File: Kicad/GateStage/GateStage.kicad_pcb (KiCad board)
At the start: 2 copper layers, 66.7 x 41.9 mm, 28 parts, among them J1 Conn_01x04, J2 Conn_01x02, J3 Conn_01x03, Q1 PHP23NQ11T,127, Q2 PHP23NQ11T,127, Q3 PHP23NQ11T,127, Q4 PHP23NQ11T,127, U1 DGD05463FN-7, U2 DGD05463FN-7

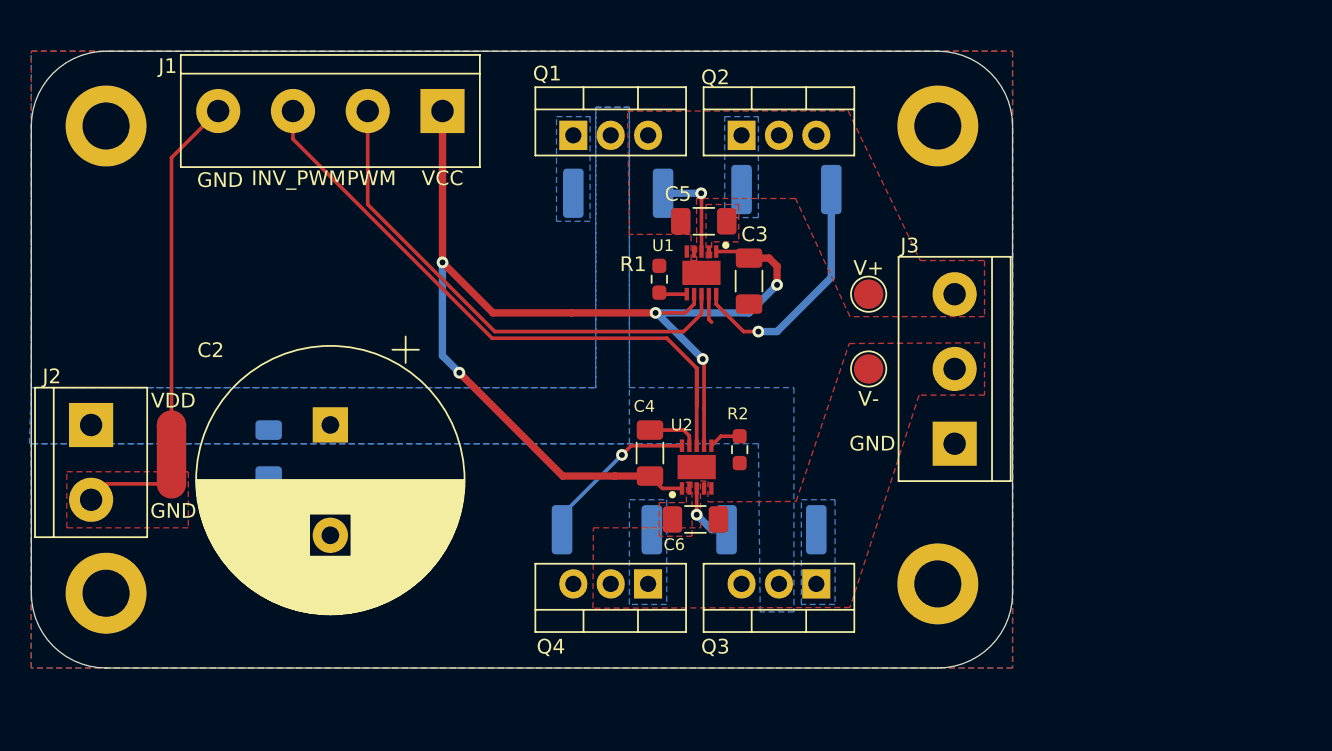
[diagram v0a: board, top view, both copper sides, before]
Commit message: Redo GateStage Board
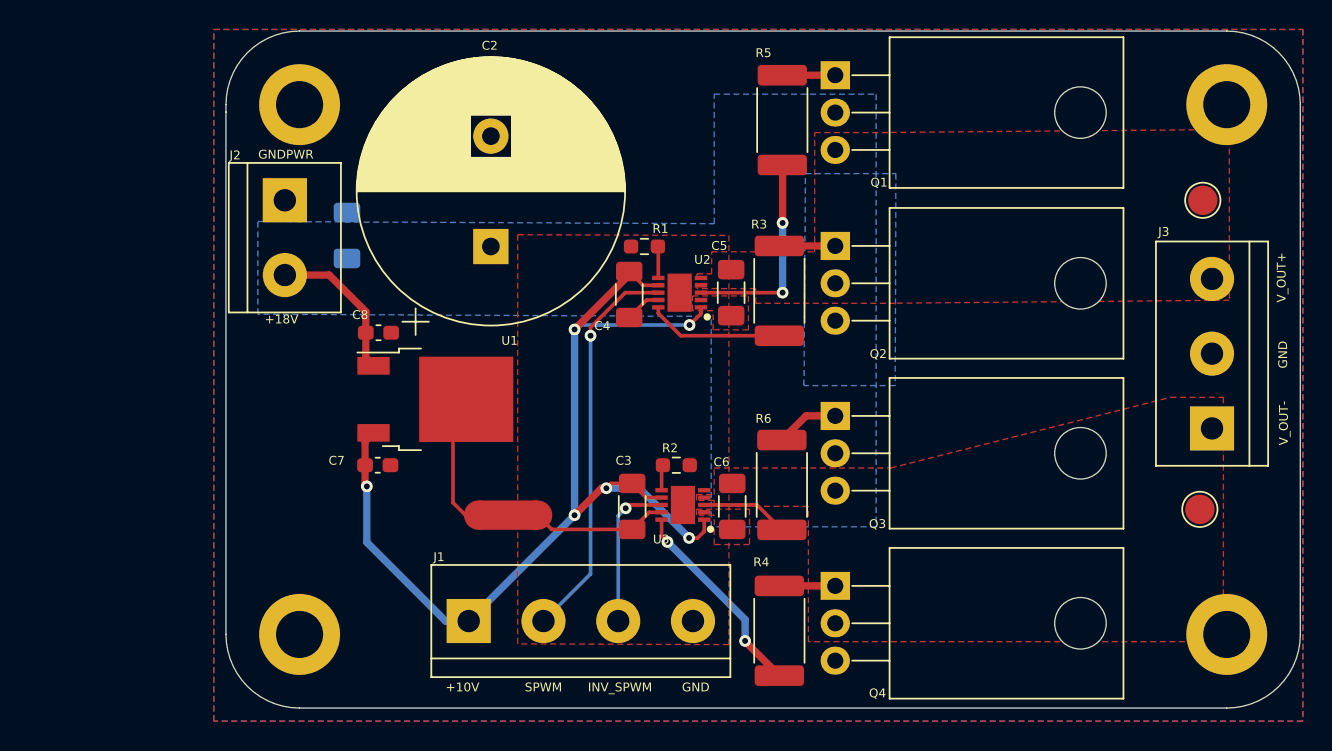
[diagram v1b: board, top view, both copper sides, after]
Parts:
- removed TPe: TestPoint, TestPoint:TestPoint_Pad_D2.0mm
- added C7: 100n, Capacitor_SMD:C_0603_1608Metric_Pad1.08x0.95mm_HandSolder, F.Cu at (125.1, 58.6)
- added C8: 330n, Capacitor_SMD:C_0603_1608Metric_Pad1.08x0.95mm_HandSolder, F.Cu at (125.2, 49.6)
- added TP2: TestPoint, TestPoint:TestPoint_Pad_D2.0mm, F.Cu at (181.0, 61.6)
- added U3: DGD05463FN-7, DGD05463:SON50P300X300X80-11N-D, F.Cu at (145.9, 61.3)
- Q1, Q2, Q3, Q4: footprint Package_TO_SOT_THT:TO-220-3_Vertical -> Package_TO_SOT_THT:TO-220-3_Horizontal_TabDown
- R3, R4, R5, R6: moved to F.Cu
- U1: value DGD05463FN-7 -> L78M10ABDT; footprint DGD05463:SON50P300X300X80-11N-D -> Package_TO_SOT_SMD:TO-252-2
- moved H2 76.2 mm to (182.8, 34.1)
- moved H1 43.4 mm to (119.8, 34.1)
- moved J1 34.7 mm to (131.3, 69.2), turned to 0 degrees
- moved TP1 23.6 mm to (181.2, 40.6)
- moved NT1 23.2 mm to (134.0, 62.0), turned to 180 degrees
- moved J2 20.2 mm to (118.8, 40.6)
- moved U1 20.0 mm to (129.1, 54.1), turned to 0 degrees
- moved H4 19.9 mm to (182.8, 70.1)
- moved Q1 18.3 mm to (156.2, 32.1), turned to 270 degrees
- moved J3 17.5 mm to (181.8, 56.1)
- moved C3 17.2 mm to (142.4, 61.4)
- moved C2 16.3 mm to (132.8, 43.8), turned to 90 degrees
- moved C1 15.7 mm to (123.0, 43.0), turned to 90 degrees
- moved R4 13.6 mm to (152.4, 69.9), turned to 270 degrees
- moved H3 13.4 mm to (119.8, 70.1)
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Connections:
- J2 pad 1: VDD -> GNDPWR
- J2 pad 2: GNDPWR -> VDD
- J3 pad 1: GNDPWR -> /H-Bridge/V_OUT-
- J3 pad 2: /H-Bridge/V_OUT- -> GNDPWR
- R3 pad 2: Net-(IC1-Pad10) -> Net-(R3-Pad2)
- R4 pad 2: Net-(IC2-Pad10) -> Net-(R4-Pad2)
- R5 pad 2: Net-(IC1-Pad3) -> Net-(R5-Pad2)
- R6 pad 2: Net-(IC2-Pad3) -> Net-(R6-Pad2)
- U1 pad 1: VCC -> VDD
- U1 pad 2: Net-(C5-Pad2) -> GNDPWR
- U1 pad 3: Net-(IC1-Pad3) -> VCC
- U2 pad 10: Net-(IC2-Pad10) -> Net-(R3-Pad2)
- U2 pad 2: Net-(C6-Pad2) -> Net-(C5-Pad2)
- U2 pad 3: Net-(IC2-Pad3) -> Net-(R5-Pad2)
- U2 pad 4: /H-Bridge/V_OUT- -> /H-Bridge/V_OUT+
- U2 pad 6: /H-Bridge/V_DT2 -> /H-Bridge/V_DT1
- U2 pad 8: /INV_PWM -> /PWM
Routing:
- net /INV_PWM: track 43.7 -> 10.4 mm, vias 0 -> 1
- net Net-(IC1-Pad10): track 16.8 -> 0.00 mm, vias 1 -> 0
- net GND: track 28.1 -> 11.8 mm
- net Net-(R5-Pad2): track 0.00 -> 14.2 mm, vias 0 -> 2
- net Net-(R4-Pad2): track 0.00 -> 13.9 mm, vias 0 -> 2
- net Net-(IC2-Pad10): track 11.1 -> 0.00 mm, vias 1 -> 0
- net VDD: track 0.00 -> 10.4 mm
- net Net-(R3-Pad2): track 0.00 -> 9.26 mm
- net VCC: track 81.4 -> 73.2 mm, vias 5 -> 6
- net /PWM: track 34.4 -> 26.9 mm, vias 0 -> 1
- net Net-(IC1-Pad3): track 6.55 -> 0.00 mm, vias 1 -> 0
- net Net-(R6-Pad2): track 0.00 -> 5.97 mm
- net Net-(Q3-Pad1): track 0.00 -> 4.31 mm
- net Net-(IC2-Pad3): track 4.24 -> 0.00 mm, vias 1 -> 0
- net Net-(Q4-Pad1): track 0.00 -> 3.80 mm
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- removed copper zone on B.Cu, net Net-(Q1-Pad1)
- removed copper zone on B.Cu, net Net-(Q2-Pad1)
- removed copper zone on B.Cu, net Net-(Q3-Pad1)
- removed copper zone on B.Cu, net Net-(Q4-Pad1)
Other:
- board size 66.7 x 41.9 mm -> 73 x 46 mm
- board text added: "+10V"
- board text added: "+18V"
- board text added: "GND"
- board text added: "GNDPWR"
- board text added: "INV_SPWM"
- board text added: "SPWM"
- board text added: "V_OUT+"
- board text added: "V_OUT-"
